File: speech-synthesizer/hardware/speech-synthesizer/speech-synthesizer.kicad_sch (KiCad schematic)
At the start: 1 part

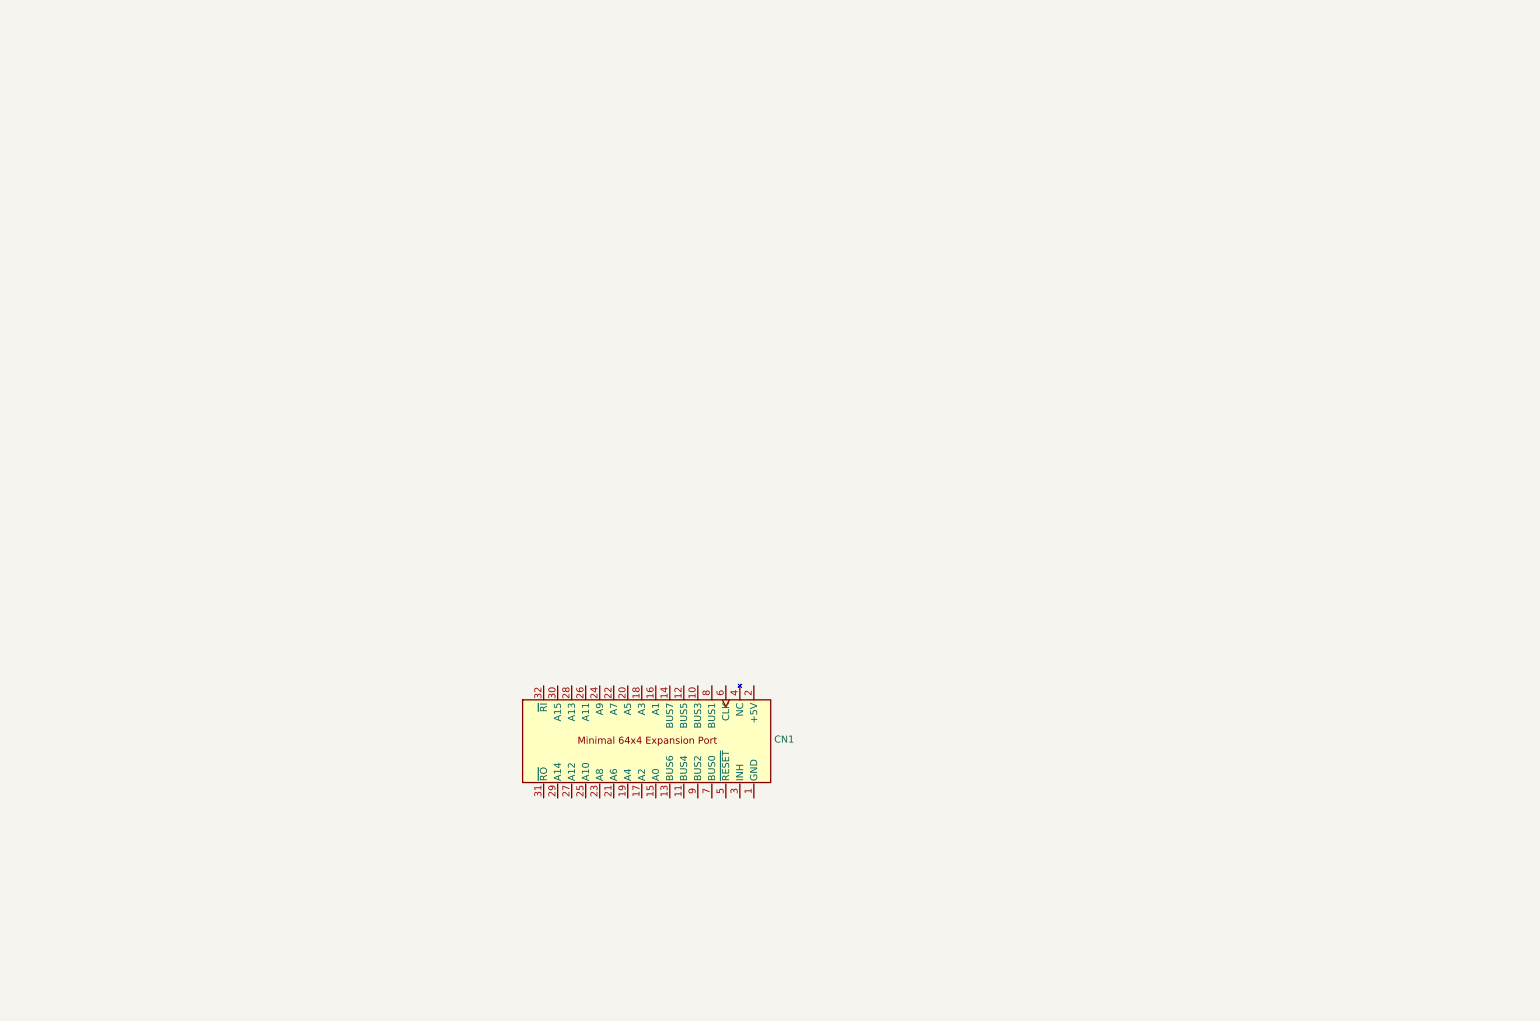
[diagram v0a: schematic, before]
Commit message: wip
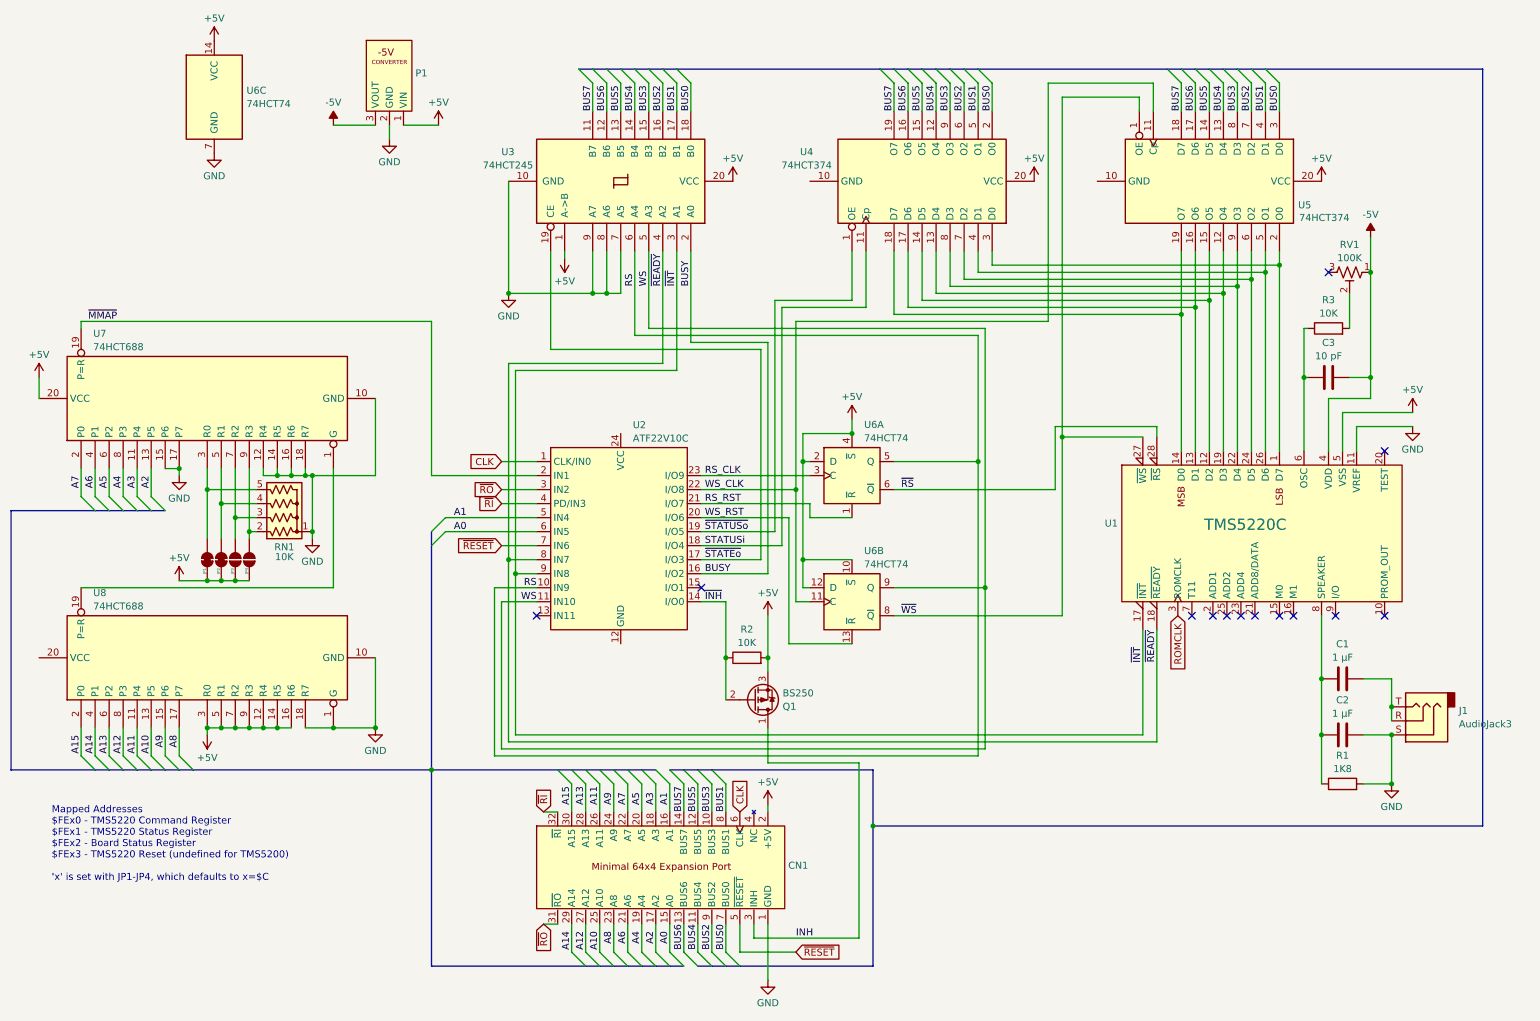
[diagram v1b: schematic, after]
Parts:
- added C1, C2: 1 µF, symbol Device:C
- added C3: 10 pF, symbol Device:C
- added J1: AudioJack3, symbol Connector_Audio:AudioJack3
- added JP1, JP2: SolderJumper_2_Bridged, symbol Jumper:SolderJumper_2_Bridged
- added JP3, JP4: SolderJumper_2_Open, symbol Jumper:SolderJumper_2_Open
- added P1: ~, symbol minimal-64x4:-5V_Converter
- added Q1: BS250, Package_TO_SOT_THT:TO-92_Inline, symbol Transistor_FET:BS250
- added R1: 1K8, symbol Device:R
- added R2, R3: 10K, symbol Device:R
- added RN1: 10K, Resistor_THT:R_Array_SIP5, symbol Device:R_Network04_US
- added RV1: 100K, symbol Device:R_Potentiometer_Trim_US
- added U1: TMS5220C, symbol minimal-64x4:TMS5220C
- added U2: ATF22V10C, symbol minimal-64x4:ATF22V10C
- added U3: 74HCT245, symbol 74xx:74HC245
- added U4, U5: 74HCT374, symbol 74xx:74HCT374
- added U6: 74HCT74, symbol 74xx:74HCT74
- added U7, U8: 74HCT688, symbol 74xx:74HCT688
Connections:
- net GND: now reaches CN1.1 (GND)
- net GND: now also C2.2, J1.S, P1.2 (GND), R1.2, RN1.1 (common), U1.11 (VREF), U3.10 (GND), U3.7 (A5), U3.8 (A6), U3.9 (A7), U6.7 (GND), U7.10 (GND), U7.12 (R4), U7.14 (R5), U7.15 (P6), U7.16 (R6), U7.17 (P7), U7.18 (R7), U8.1 (G), U8.10 (GND), U8.18 (R7)
- net BUS3: now reaches CN1.10 (BUS3)
- net BUS3: now also U3.15 (B3), U4.9 (O3), U5.8 (D3)
- net BUS4: now reaches CN1.11 (BUS4)
- net BUS4: now also U3.14 (B4), U4.12 (O4), U5.13 (D4)
- net BUS5: now reaches CN1.12 (BUS5)
- net BUS5: now also U3.13 (B5), U4.15 (O5), U5.14 (D5)
- net BUS6: now reaches CN1.13 (BUS6)
- net BUS6: now also U3.12 (B6), U4.16 (O6), U5.17 (D6)
- net BUS7: now reaches CN1.14 (BUS7)
- net BUS7: now also U3.11 (B7), U4.19 (O7), U5.18 (D7)
- net A0: now reaches CN1.15 (A0)
- net A0: now also U2.6 (IN5)
- net A1: now reaches CN1.16 (A1)
- net A1: now also U2.5 (IN4)
- net A2: now reaches CN1.17 (A2)
- net A2: now also U7.13 (P5)
- net A3: now reaches CN1.18 (A3)
- net A3: now also U7.11 (P4)
- net A4: now reaches CN1.19 (A4)
- net A4: now also U7.8 (P3)
- net +5V: now reaches CN1.2 (+5V)
- net +5V: now also JP1.1 (A), JP2.1 (A), JP3.1 (A), JP4.1 (A), P1.1 (VIN), Q1.3 (S), R2.2, U1.5 (VSS), U3.1 (A->B), U3.20 (VCC), U4.20 (VCC), U5.20 (VCC), U6.10 (~{S}), U6.12 (D), U6.14 (VCC), U6.2 (D), U6.4 (~{S}), U7.20 (VCC), U8.12 (R4), U8.14 (R5), U8.16 (R6), U8.3 (R0), U8.5 (R1), U8.7 (R2), U8.9 (R3)
- net A5: now reaches CN1.20 (A5)
- net A5: now also U7.6 (P2)
- net A6: now reaches CN1.21 (A6)
- net A6: now also U7.4 (P1)
- net A7: now reaches CN1.22 (A7)
- net A7: now also U7.2 (P0)
- net A8: now reaches CN1.23 (A8)
- net A8: now also U8.17 (P7)
- net A9: now reaches CN1.24 (A9)
- net A9: now also U8.15 (P6)
- net A10: now reaches CN1.25 (A10)
- net A10: now also U8.13 (P5)
- net A11: now reaches CN1.26 (A11)
- net A11: now also U8.11 (P4)
- net A12: now reaches CN1.27 (A12)
- net A12: now also U8.8 (P3)
- net A13: now reaches CN1.28 (A13)
- net A13: now also U8.6 (P2)
- net A14: now reaches CN1.29 (A14)
- net A14: now also U8.4 (P1)
- net INH: now reaches CN1.3 (INH)
- net INH: now also Q1.1 (D)
- net A15: now reaches CN1.30 (A15)
- net A15: now also U8.2 (P0)
- net ~{RO}: now reaches CN1.31 (~{RO})
- net ~{RO}: now also U2.3 (IN2)
- net ~{RI}: now reaches CN1.32 (~{RI})
- net ~{RI}: now also U2.4 (PD/IN3)
- net ~{RESET}: now reaches CN1.5 (~{RESET})
- net ~{RESET}: now also U2.7 (IN6)
- net CLK: now reaches CN1.6 (CLK)
- net CLK: now also U2.1 (CLK/IN0)
- net BUS0: now reaches CN1.7 (BUS0)
- net BUS0: now also U3.18 (B0), U4.2 (O0), U5.3 (D0)
- net BUS1: now reaches CN1.8 (BUS1)
- net BUS1: now also U3.17 (B1), U4.5 (O1), U5.4 (D1)
- net BUS2: now reaches CN1.9 (BUS2)
- net BUS2: now also U3.16 (B2), U4.6 (O2), U5.7 (D2)
- new net: U7.1 (G), U8.19 (P=R)
- new net: JP1.2 (B), RN1.5 (R4), U7.3 (R0)
- new net: JP2.2 (B), RN1.4 (R3), U7.5 (R1)
- new net: JP3.2 (B), RN1.3 (R2), U7.7 (R2)
- new net: JP4.2 (B), RN1.2 (R1), U7.9 (R3)
- new net: C1.2, J1.R, J1.T
- new net: U1.1 (D7), U4.3 (D0), U5.2 (O0)
- new net: U1.12 (D2), U4.14 (D5), U5.15 (O5)
- new net: U1.13 (D1), U4.17 (D6), U5.16 (O6)
- new net: U1.14 (D0), U4.18 (D7), U5.19 (O7)
- new net: U1.19 (D3), U4.13 (D4), U5.12 (O4)
- new net: U1.22 (D4), U4.8 (D3), U5.9 (O3)
- new net: U1.24 (D5), U4.7 (D2), U5.6 (O2)
- new net: U1.26 (D6), U4.4 (D1), U5.5 (O1)
- new net: C3.2, R3.1, U1.6 (OSC)
- new net: C1.1, C2.1, R1.1, U1.8 (SPEAKER)
- new net: R3.2, RV1.2
- new net -5V: C3.1, P1.3 (VOUT), RV1.1, U1.4 (VDD)
- new net BUSY: U2.16 (I/O2), U3.2 (A0)
- new net ROMCLK: U1.3 (ROMCLK)
- new net RS: U2.10 (IN9), U3.6 (A4), U6.5 (Q)
- new net RS_CLK: U2.23 (I/O9), U6.3 (C)
- new net RS_RST: U2.21 (I/O7), U6.1 (~{R})
- new net STATUSi: U2.18 (I/O4), U4.11 (Cp)
- new net WS: U2.11 (IN10), U3.5 (A3), U6.9 (Q)
- new net WS_CLK: U2.22 (I/O8), U5.11 (Cp), U6.11 (C)
- new net WS_RST: U2.20 (I/O6), U6.13 (~{R})
- new net ~{INH}: Q1.2 (G), R2.1, U2.14 (I/O0)
- new net ~{INT}: U1.17 (~{INT}), U2.9 (IN8), U3.3 (A1)
- new net ~{MMAP}: U2.2 (IN1), U7.19 (P=R)
- new net ~{READY}: U1.18 (~{READY}), U2.8 (IN7), U3.4 (A2)
- new net ~{RS}: U1.28 (~{RS}), U6.6 (~{Q})
- new net ~{STATEo}: U2.17 (I/O3), U3.19 (CE)
- new net ~{STATUSo}: U2.19 (I/O5), U4.1 (OE)
- new net ~{WS}: U1.27 (~{WS}), U5.1 (OE), U6.8 (~{Q})
- no-connect marks 0 -> 13
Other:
- note added: "Mapped Addresses $FEx0 - TMS5220 Command Register $FEx1 - TMS5220 Status Register $FEx2 - Board Status Register $FEx3 - TMS5220 Reset (undefined for TMS5200) 'x' is set with JP1-JP4, which defaults to x=$C"
- moved on the sheet: CN1
